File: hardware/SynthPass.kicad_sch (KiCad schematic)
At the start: 14 parts, among them J1 SM04B-SRSS-TB, P1 USB_C_Plug_USB2.0, SW1 SW_Push, U2 CH572D, Y2 32MHz

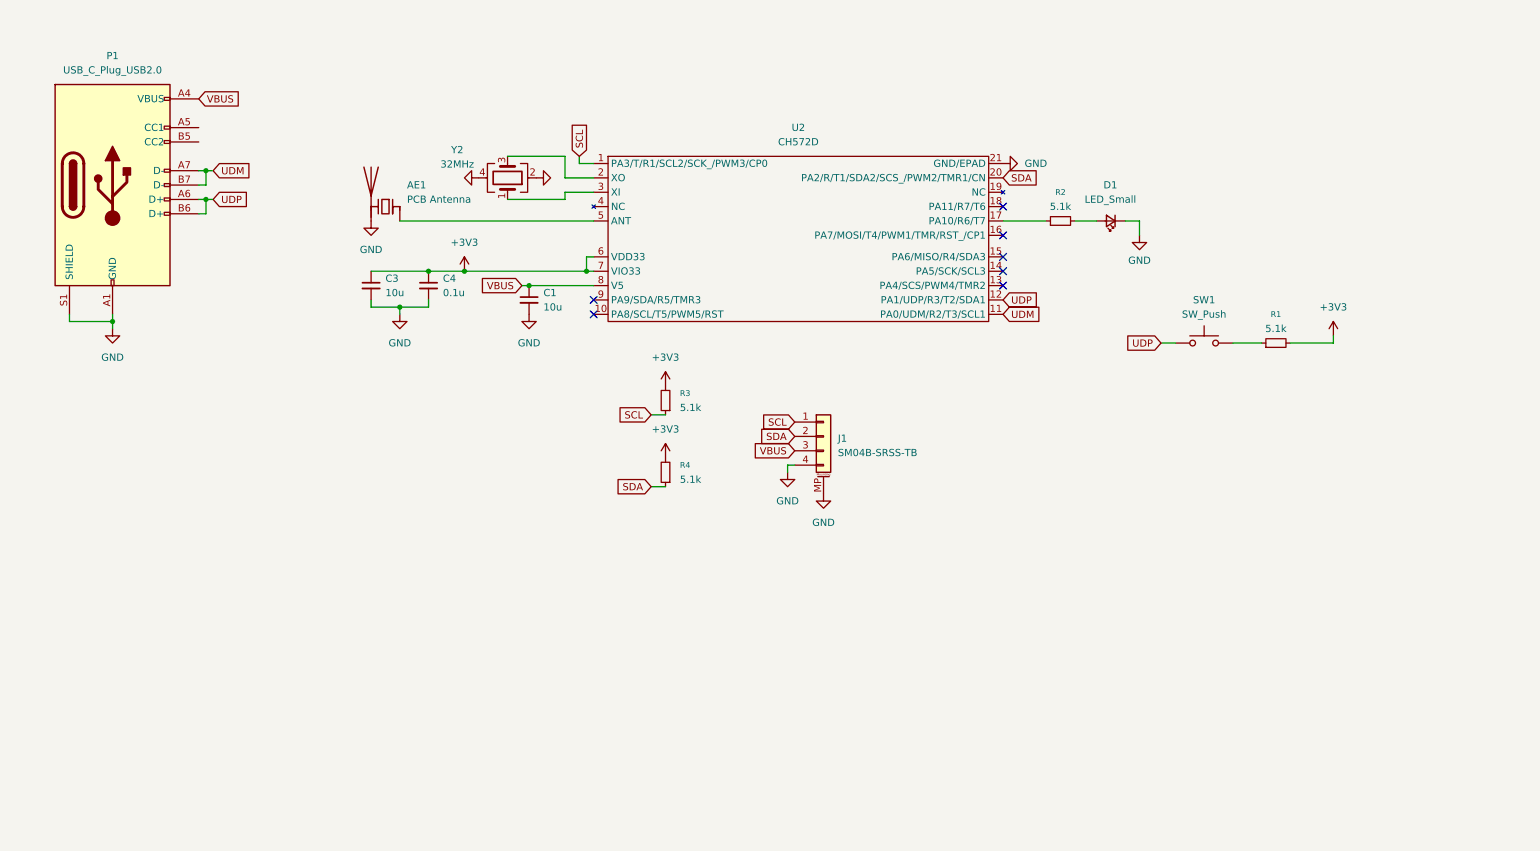
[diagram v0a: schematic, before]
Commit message: v2 schematic changes pending review
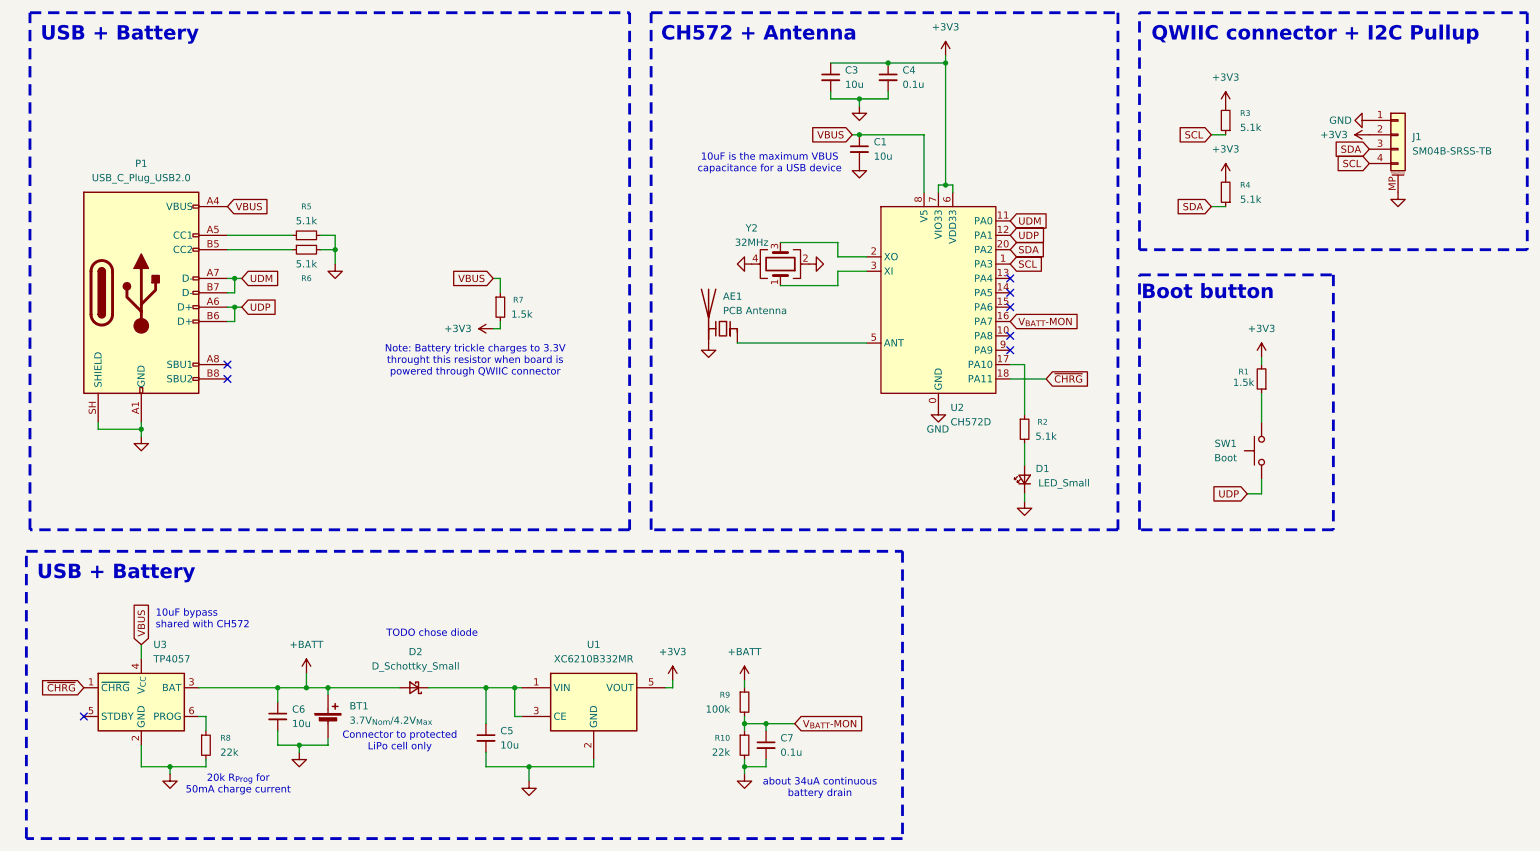
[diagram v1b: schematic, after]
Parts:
- added BT1: 3.7V_{Nom}/4.2V_{Max}, symbol Device:Battery_Cell
- added C5, C6: 10u, Capacitor_SMD:C_0402_1005Metric, symbol Device:C_Small
- added C7: 0.1u, Capacitor_SMD:C_0402_1005Metric, symbol Device:C_Small
- added D2: D_Schottky_Small, symbol Device:D_Schottky_Small
- added R10, R8: 22k, symbol Device:R_Small
- added R5, R6: 5.1k, symbol Device:R_Small
- added R7: 1.5k, Resistor_SMD:R_0402_1005Metric, symbol Device:R_Small
- added R9: 100k, symbol Device:R_Small
- added U1: XC6210B332MR, Package_TO_SOT_SMD:SOT-23-5, symbol Regulator_Linear:XC6210B332MR
- added U3: TP4057, Package_TO_SOT_SMD:TSOT-23-6, symbol Battery_Management:TP4057
- P1: symbol Connector:USB_C_Receptacle_USB2.0_14P -> Connector:USB_C_Receptacle_USB2.0_16P
- R1: value 5.1k -> 1.5k
- SW1: value SW_Push -> Boot
- U2: footprint CH572D:CH572D -> Ch572D:CH572D; symbol CH572D:CH572D -> CH572D:CH572D_small
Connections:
- net +3V3: now also J1.2 (Pin_2), R7.2, U1.5 (VOUT)
- net GND: now also J1.1 (Pin_1), P1.SH (SHIELD), U2.0 (GND), BT1.2 (-), C5.2, C6.2, C7.2, R10.2, R5.2, R6.2, R8.2, U1.2 (GND), U3.2 (GND); no longer J1.4 (Pin_4), P1.S1 (SHIELD), U2.21 (GND/EPAD)
- net SCL: now also J1.4 (Pin_4); no longer J1.1 (Pin_1)
- net SDA: now also J1.3 (Pin_3); no longer J1.2 (Pin_2)
- net VBUS: now also R7.1, U3.4 (V_{CC}); no longer J1.3 (Pin_3)
- net at P1.A5 (CC1): now also R5.1
- net at P1.B5 (CC2): now also R6.1
- net V_{BATT}-MON: now reaches U2.16 (PA7)
- net V_{BATT}-MON: now also C7.1, R10.1, R9.2
- net ~{CHRG}: now reaches U2.18 (PA11)
- net ~{CHRG}: now also U3.1 (~{CHRG})
- net at U2.19 (NC): now also U2.4 (NC)
- new net: R8.1, U3.6 (PROG)
- new net: C5.1, D2.1 (K), U1.1 (VIN), U1.3 (CE)
- new net +BATT: BT1.1 (+), C6.1, D2.2 (A), R9.1, U3.3 (BAT)
- no-connect marks 7 -> 8
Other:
- note added: "10uF bypass shared with CH572"
- note added: "10uF is the maximum VBUS capacitance for a USB device"
- note added: "20k R_{Prog} for 50mA charge current"
- note added: "Boot button"
- note added: "CH572 + Antenna"
- note added: "Connector to protected LiPo cell only"
- note added: "Note: Battery trickle charges to 3.3V throught this resistor when board is powered through QWIIC connector"
- note added: "QWIIC connector + I2C Pullup"
- note added: "TODO chose diode"
- note added: "USB + Battery"
- note added: "about 34uA continuous battery drain"
- moved on the sheet: AE1, C1, C3, C4, D1, J1, R1, R2, R3, R4, SW1, Y2
